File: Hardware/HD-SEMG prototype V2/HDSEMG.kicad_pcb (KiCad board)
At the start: 2 copper layers, 150 x 86.9 mm, 210 parts, among them IC1 ADS1298_By_Oliver, J1 AUDIO_JACK_By_OLIVER, J10 Conn_01x02, J11 Barrel_Jack_Switch, J12 Conn_01x01, J13 Conn_01x03, J14 Conn_01x03, J15 Conn_01x03, J16 Conn_01x03, J17 Conn_01x03, J18 AUDIO_JACK_By_OLIVER, J19 Conn_01x06, J2 Conn_01x04, J21 Conn_01x03, J22 Conn_01x03, J23 Conn_01x03, J24 Conn_01x03, J25 Conn_01x03, J26 Conn_01x03, J3 Conn_02x02_Counter_Clockwise, J30 Conn_01x08, J31 Screw_Terminal_01x02, J4 Conn_02x02_Counter_Clockwise, J5 Conn_02x02_Counter_Clockwise, J7 Conn_01x01, J8 Conn_01x01, J9 Conn_01x02, U10 OPA333xxDBV, U11 TLV1117-25, U12 MCP1825S, U13 MAX889TESA+, U14 TPS72325, U15 INA333AIDGKR, U16 OPA333xxDBV, U17 THS4521IDGKT, U2 Si8663, U3 Si8663, U33 INA333AIDGKR, U34 OPA333xxDBV, U35 THS4521IDGKT, U36 357LB3CI002M0480, U8 INA333AIDGKR, U9 THS4521IDGKT

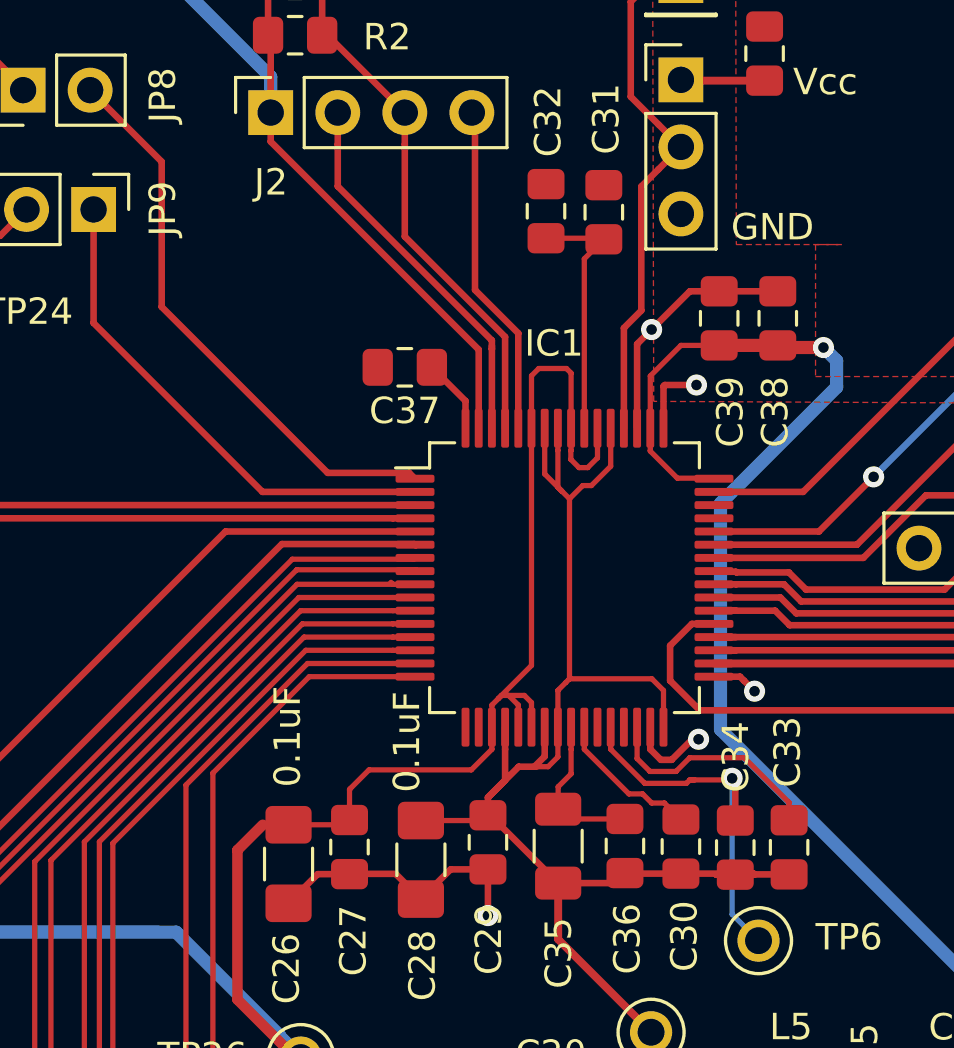
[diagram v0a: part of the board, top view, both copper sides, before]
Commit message: update
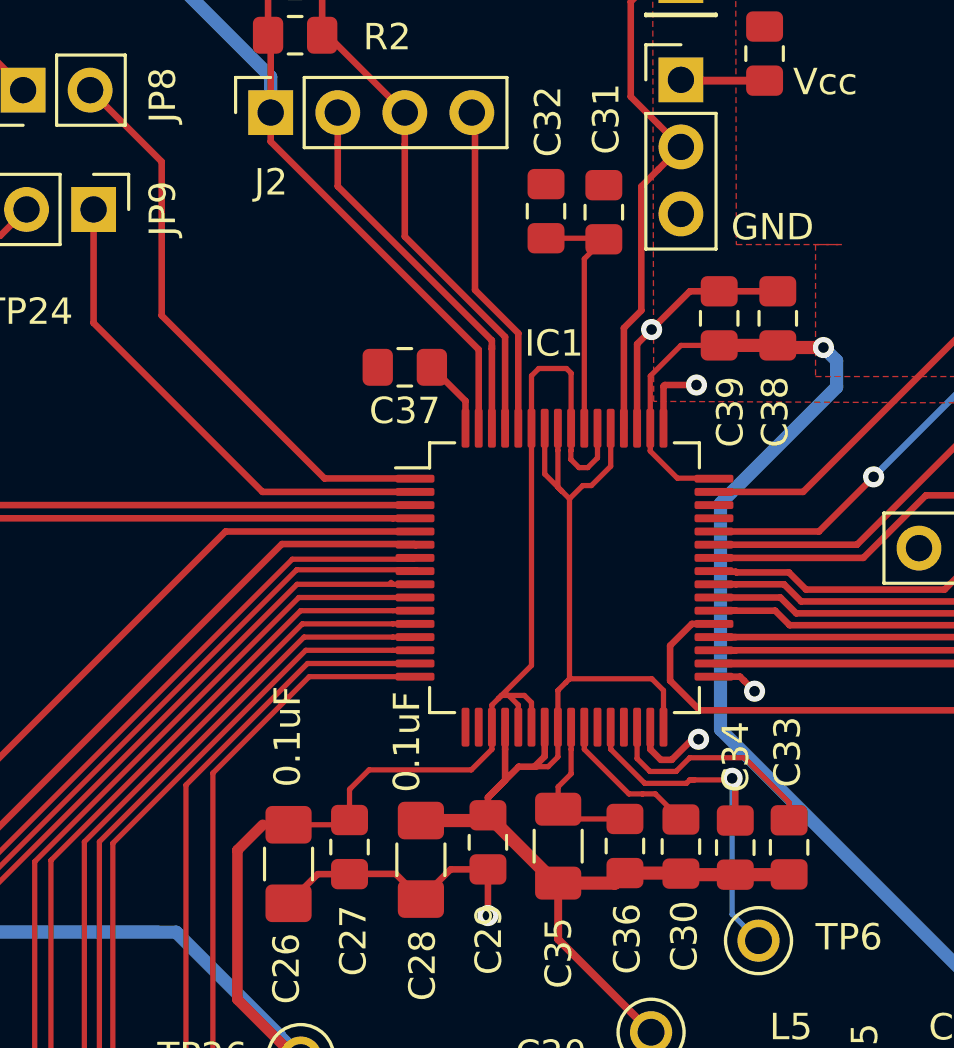
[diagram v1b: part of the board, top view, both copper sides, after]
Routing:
- net -2V5: track 113.2 -> 117.3 mm
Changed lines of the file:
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@@
     (thickness 1.6)
     (drawings 47)
-    (tracks 1255)
+    (tracks 1258)
     (zones 0)
     (modules 210)
@@
   )
   (setup
-    (last_trace_width 0.4)
+    (last_trace_width 0.5)
     (user_trace_width 0.2)
     (user_trace_width 0.3)
@@
   (segment (start 113.77 96.45) (end 113.77 95.3425) (width 0.25) (layer F.Cu) (net 13) (status 20))
   (segment (start 113.38 96.84) (end 113.77 96.45) (width 0.25) (layer F.Cu) (net 13))
-  (segment (start 111.42 98.88) (end 111.62 98.68) (width 0.2) (layer F.Cu) (net 13) (status 30))
-  (segment (start 109.08 98.88) (end 111.42 98.88) (width 0.2) (layer F.Cu) (net 13) (status 30))
   (segment (start 118.27 93.95) (end 118.27 95.3425) (width 0.2) (layer F.Cu) (net 13) (status 20))
   (segment (start 117.83 93.51) (end 118.27 93.95) (width 0.2) (layer F.Cu) (net 13))
@@
   (segment (start 121.72 100.92) (end 120.26 100.92) (width 0.25) (layer F.Cu) (net 13))
   (segment (start 123.03 100.92) (end 121.72 100.92) (width 0.25) (layer F.Cu) (net 13) (status 10))
-  (segment (start 116.83 100.89) (end 116.81 100.87) (width 0.25) (layer F.Cu) (net 13) (status 30))
-  (segment (start 118.93 100.89) (end 116.83 100.89) (width 0.25) (layer F.Cu) (net 13) (status 30))
-  (segment (start 111.71 98.68) (end 111.62 98.68) (width 0.25) (layer F.Cu) (net 13) (status 30))
-  (segment (start 114.28 101.25) (end 111.71 98.68) (width 0.25) (layer F.Cu) (net 13) (status 30))
   (segment (start 107.375 81.78) (end 107.445 81.71) (width 0.2) (layer F.Cu) (net 13) (status 30))
   (via (at 78.34 87.93) (size 0.8) (drill 0.4) (layers F.Cu B.Cu) (net 13))
@@
   (segment (start 43.9 74.25) (end 43.9 74.8) (width 0.25) (layer F.Cu) (net 13))
   (segment (start 43.9 74.8) (end 44.83 75.73) (width 0.25) (layer F.Cu) (net 13))
-  (segment (start 116.43 101.25) (end 116.81 100.87) (width 0.25) (layer F.Cu) (net 13) (status 30))
-  (segment (start 114.28 101.25) (end 116.43 101.25) (width 0.25) (layer F.Cu) (net 13) (status 30))
   (via (at 78.33 102.26) (size 0.8) (drill 0.4) (layers F.Cu B.Cu) (net 13))
   (segment (start 77.54 100.48) (end 77.54 101.47) (width 0.25) (layer F.Cu) (net 13))
@@
   (segment (start 114.28 103.38) (end 114.28 101.25) (width 0.3) (layer F.Cu) (net 13))
   (segment (start 117.8 106.9) (end 114.28 103.38) (width 0.3) (layer F.Cu) (net 13))
+  (segment (start 114.19 101.25) (end 111.62 98.68) (width 0.5) (layer F.Cu) (net 13))
+  (segment (start 114.28 101.25) (end 114.19 101.25) (width 0.5) (layer F.Cu) (net 13))
+  (segment (start 111.42 98.88) (end 111.62 98.68) (width 0.5) (layer F.Cu) (net 13))
+  (segment (start 109.08 98.88) (end 111.42 98.88) (width 0.5) (layer F.Cu) (net 13))
+  (segment (start 116.43 101.25) (end 116.81 100.87) (width 0.5) (layer F.Cu) (net 13))
+  (segment (start 114.28 101.25) (end 116.43 101.25) (width 0.5) (layer F.Cu) (net 13))
+  (segment (start 118.91 100.87) (end 118.93 100.89) (width 0.5) (layer F.Cu) (net 13))
+  (segment (start 116.81 100.87) (end 118.91 100.87) (width 0.5) (layer F.Cu) (net 13))
+  (segment (start 123.02 100.93) (end 123.03 100.92) (width 0.5) (layer F.Cu) (net 13))
+  (segment (start 120.99 100.93) (end 123.02 100.93) (width 0.5) (layer F.Cu) (net 13))
+  (segment (start 118.97 100.93) (end 118.93 100.89) (width 0.5) (layer F.Cu) (net 13))
+  (segment (start 120.99 100.93) (end 118.97 100.93) (width 0.5) (layer F.Cu) (net 13))
   (segment (start 83.51501 67.90499) (end 85.61499 67.90499) (width 0.25) (layer F.Cu) (net 14))
   (segment (start 87.79 68.93) (end 86.64 68.93) (width 0.25) (layer F.Cu) (net 14) (status 20))
@@
   (segment (start 128.638 110.5) (end 128.572 110.566) (width 0.25) (layer F.Cu) (net 27) (status 30))
   (segment (start 128.53 108.46) (end 128.53 110.6) (width 0.25) (layer F.Cu) (net 27) (status 30))
-  (segment (start 117.478278 97.870734) (end 116.960734 97.870734) (width 0.2) (layer F.Cu) (net 28))
-  (segment (start 115.27 96.18) (end 115.27 95.3425) (width 0.2) (layer F.Cu) (net 28) (status 20))
-  (segment (start 118.93 98.84) (end 118.306628 98.216628) (width 0.2) (layer F.Cu) (net 28) (status 10))
-  (segment (start 118.306628 98.216628) (end 117.824172 98.216628) (width 0.2) (layer F.Cu) (net 28))
+  (segment (start 115.27 96.18) (end 115.27 95.3425) (width 0.2) (layer F.Cu) (net 28))
   (segment (start 116.960734 97.870734) (end 115.27 96.18) (width 0.2) (layer F.Cu) (net 28))
-  (segment (start 117.824172 98.216628) (end 117.478278 97.870734) (width 0.2) (layer F.Cu) (net 28))
+  (segment (start 117.478278 97.870734) (end 116.960734 97.870734) (width 0.2) (layer F.Cu) (net 28))
+  (segment (start 117.479012 97.87) (end 117.478278 97.870734) (width 0.2) (layer F.Cu) (net 28))
+  (segment (start 118.93 98.84) (end 117.96 97.87) (width 0.2) (layer F.Cu) (net 28))
+  (segment (start 117.96 97.87) (end 117.479012 97.87) (width 0.2) (layer F.Cu) (net 28))
   (segment (start 115.27 77.6) (end 116.01 76.86) (width 0.2) (layer F.Cu) (net 29) (status 20))
   (segment (start 115.27 84.0175) (end 115.27 77.6) (width 0.2) (layer F.Cu) (net 29) (status 10))
@@
   (segment (start 120.87 102.43) (end 121.87 103.43) (width 0.2) (layer B.Cu) (net 31) (status 20))
   (segment (start 120.87 97.28) (end 120.87 102.43) (width 0.2) (layer B.Cu) (net 31))
-  (segment (start 116.27 96.18) (end 116.27 95.3425) (width 0.2) (layer F.Cu) (net 31) (status 20))
-  (segment (start 117.560723 97.470723) (end 116.27 96.18) (width 0.2) (layer F.Cu) (net 31))
-  (segment (start 119.27 97.340011) (end 119.139288 97.470723) (width 0.2) (layer F.Cu) (net 31))
-  (segment (start 119.139288 97.470723) (end 117.560723 97.470723) (width 0.2) (layer F.Cu) (net 31))
   (segment (start 120.99 97.4) (end 120.87 97.28) (width 0.25) (layer F.Cu) (net 31))
   (segment (start 120.99 98.88) (end 120.99 97.4) (width 0.25) (layer F.Cu) (net 31) (status 10))
+  (segment (start 117.559989 97.469989) (end 116.27 96.18) (width 0.2) (layer F.Cu) (net 31))
+  (segment (start 119.140022 97.469989) (end 117.559989 97.469989) (width 0.2) (layer F.Cu) (net 31))
+  (segment (start 119.27 97.340011) (end 119.140022 97.469989) (width 0.2) (layer F.Cu) (net 31))
+  (segment (start 116.27 96.18) (end 116.27 95.3425) (width 0.2) (layer F.Cu) (net 31))
   (segment (start 114.77 96.18) (end 114.77 95.3425) (width 0.2) (layer F.Cu) (net 32) (status 20))
   (segment (start 114.77 97.110346) (end 114.77 96.18) (width 0.2) (layer F.Cu) (net 32))
@@
   (segment (start 96.68 80.03) (end 96.68 75.73) (width 0.25) (layer F.Cu) (net 73))
   (segment (start 103.08 86.43) (end 96.68 80.03) (width 0.25) (layer F.Cu) (net 73))
-  (segment (start 108.63679 85.70929) (end 105.54929 85.70929) (width 0.25) (layer F.Cu) (net 74))
-  (segment (start 108.8575 85.93) (end 108.63679 85.70929) (width 0.25) (layer F.Cu) (net 74))
-  (segment (start 105.54929 85.70929) (end 99.26 79.42) (width 0.25) (layer F.Cu) (net 74))
   (segment (start 99.26 73.92) (end 96.55 71.21) (width 0.25) (layer F.Cu) (net 74))
-  (segment (start 99.26 79.42) (end 99.26 73.92) (width 0.25) (layer F.Cu) (net 74))
+  (segment (start 99.26 79.75) (end 99.26 73.92) (width 0.25) (layer F.Cu) (net 74))
+  (segment (start 108.63679 85.92) (end 105.43 85.92) (width 0.25) (layer F.Cu) (net 74))
+  (segment (start 105.43 85.92) (end 99.26 79.75) (width 0.25) (layer F.Cu) (net 74))
   (segment (start 131.821765 92.93) (end 120.1825 92.93) (width 0.3) (layer F.Cu) (net 75))
   (segment (start 140.632081 84.76) (end 141.93 86.057919) (width 0.3) (layer F.Cu) (net 75))
@@
   (segment (start 140.279999 77.989999) (end 147.092881 77.989999) (width 0.3) (layer F.Cu) (net 91))
   (segment (start 139.43 77.14) (end 140.279999 77.989999) (width 0.3) (layer F.Cu) (net 91))
-  (segment (start 137.16 102.58) (end 134.27 99.69) (width 0.25) (layer F.Cu) (net 139))
-  (segment (start 139.3 102.58) (end 137.16 102.58) (width 0.25) (layer F.Cu) (net 139) (status 10))
-  (segment (start 139.3 102.23) (end 139.3 102.58) (width 0.25) (layer F.Cu) (net 139) (status 30))
-  (segment (start 140.69 100.84) (end 139.3 102.23) (width 0.25) (layer F.Cu) (net 139) (status 20))
-  (segment (start 143.03 100.84) (end 140.69 100.84) (width 0.25) (layer F.Cu) (net 139) (status 10))
-  (segment (start 134.27 99.69) (end 134.27 98.59) (width 0.25) (layer F.Cu) (net 139))
   (segment (start 41.555002 101.789998) (end 41.565 101.78) (width 0.25) (layer F.Cu) (net 92) (status 30))
   (segment (start 37.62 116.22) (end 37.61 116.23) (width 0.25) (layer F.Cu) (net 92))
@@
   (segment (start 162.83 79.66) (end 162.78 79.61) (width 0.3) (layer F.Cu) (net 138))
   (segment (start 166.53 79.66) (end 162.83 79.66) (width 0.3) (layer F.Cu) (net 138))
+  (segment (start 137.16 102.58) (end 134.27 99.69) (width 0.25) (layer F.Cu) (net 139))
+  (segment (start 139.3 102.58) (end 137.16 102.58) (width 0.25) (layer F.Cu) (net 139) (status 10))
+  (segment (start 139.3 102.23) (end 139.3 102.58) (width 0.25) (layer F.Cu) (net 139) (status 30))
+  (segment (start 140.69 100.84) (end 139.3 102.23) (width 0.25) (layer F.Cu) (net 139) (status 20))
+  (segment (start 143.03 100.84) (end 140.69 100.84) (width 0.25) (layer F.Cu) (net 139) (status 10))
+  (segment (start 134.27 99.69) (end 134.27 98.59) (width 0.25) (layer F.Cu) (net 139))
   (segment (start 49.04 62.5) (end 48.94 62.4) (width 0.4) (layer F.Cu) (net 140))
   (segment (start 54.25 62.5) (end 49.04 62.5) (width 0.4) (layer F.Cu) (net 140))
